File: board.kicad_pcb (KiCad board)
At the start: 2 copper layers, 135 x 100 mm, 12 parts, among them J1 Conn_01x02, J2 Conn_01x02, J3 Conn_01x02

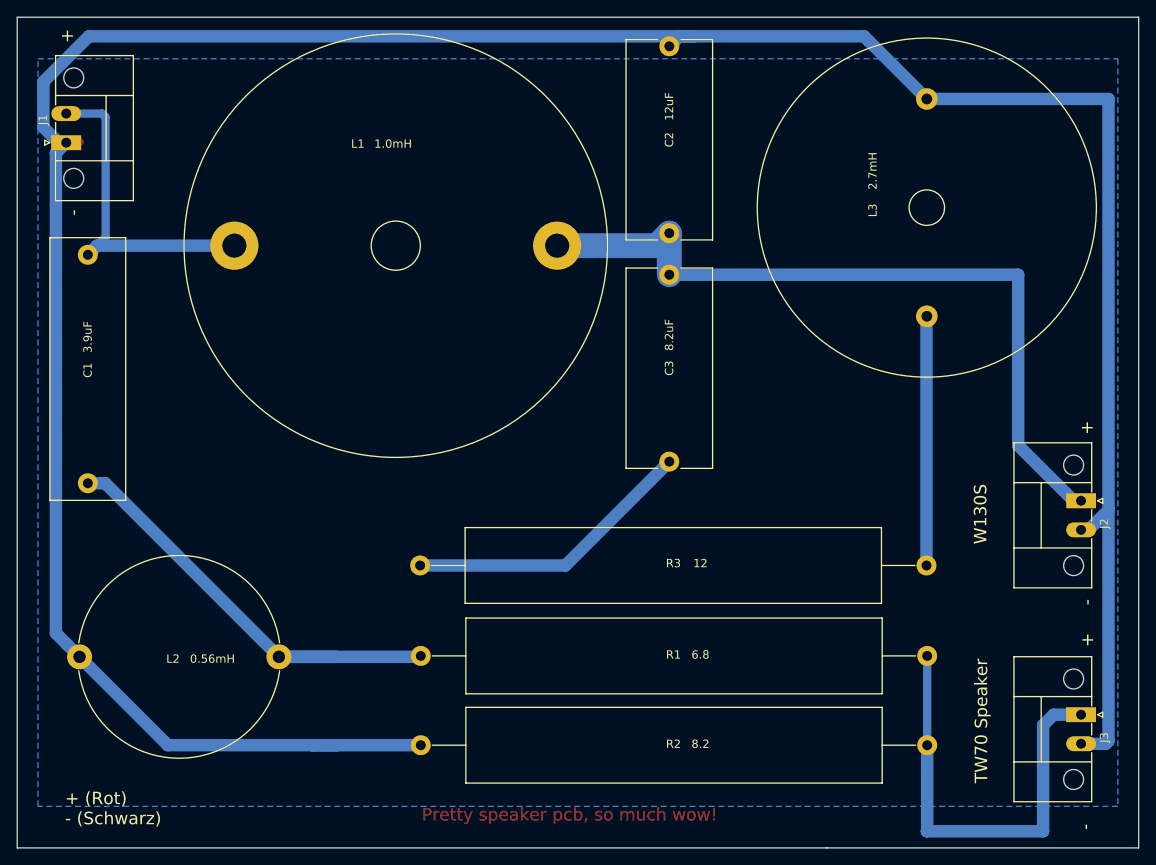
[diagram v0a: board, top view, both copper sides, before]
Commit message: Syncing AISLER project with GitHub repository
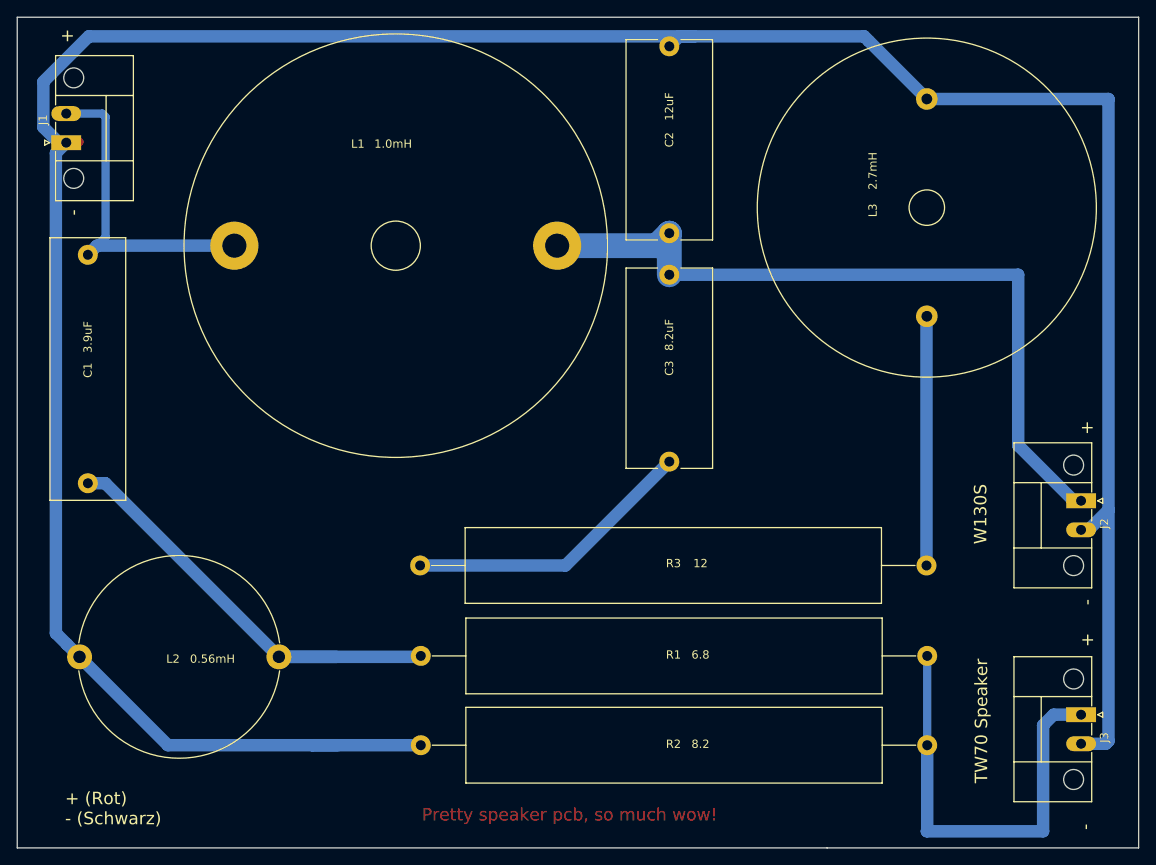
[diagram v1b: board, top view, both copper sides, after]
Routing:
- removed copper zone on B.Cu, net (none)
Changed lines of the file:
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@@
   (segment (start 124.5 82.5) (end 126 81) (width 3) (layer B.Cu) (net 7))
   (segment (start 126 86) (end 126 81) (width 3) (layer B.Cu) (net 7))
-  (zone (net 0) (net_name "") (layer B.Cu) (hatch edge 0.508)
-    (connect_pads (clearance 0.508))
-    (min_thickness 0.254)
-    (fill yes (arc_segments 16) (thermal_gap 0.508) (thermal_bridge_width 0.508))
-    (polygon
-      (pts
-        (xy 50 60) (xy 180 60) (xy 180 150) (xy 50 150)
-      )
-    )
-  )
 )

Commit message: Syncing AISLER project with GitHub repository
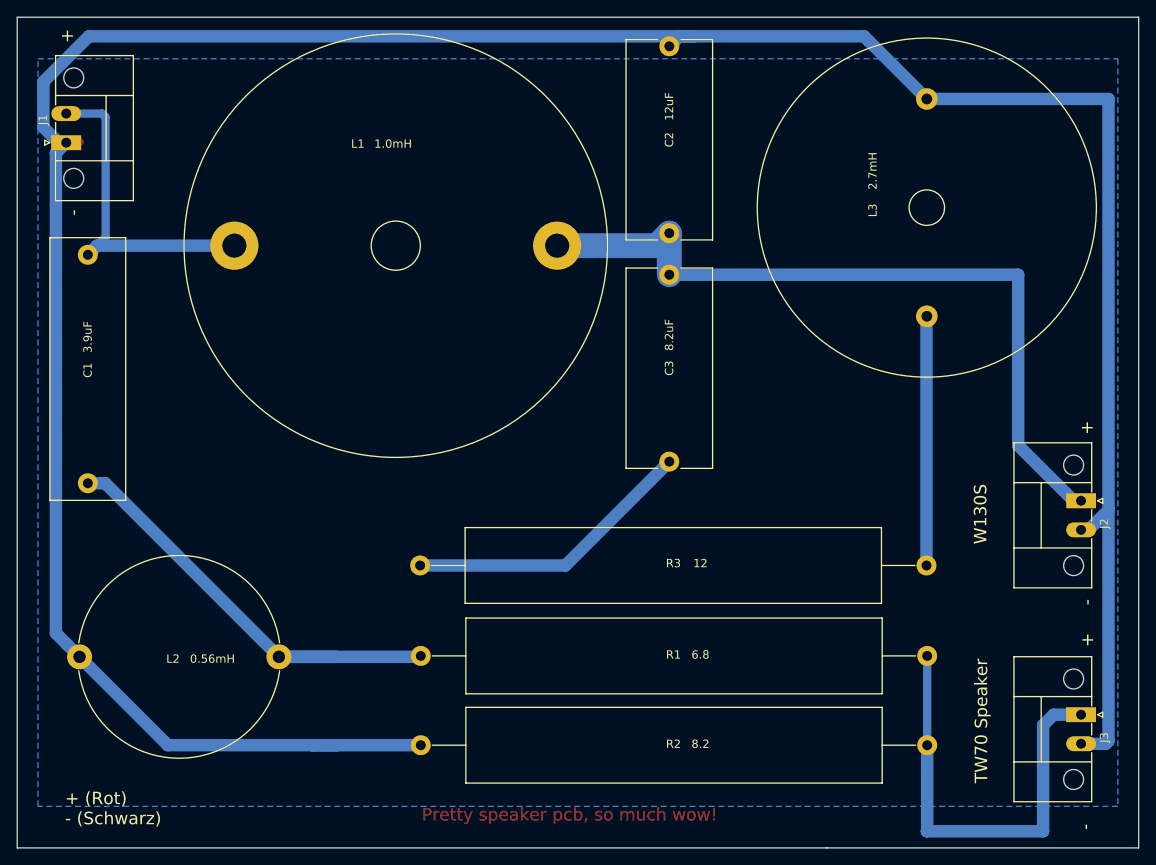
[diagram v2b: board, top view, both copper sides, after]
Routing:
- added copper zone on B.Cu, net (none)
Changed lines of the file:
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@@
   (segment (start 124.5 82.5) (end 126 81) (width 3) (layer B.Cu) (net 7))
   (segment (start 126 86) (end 126 81) (width 3) (layer B.Cu) (net 7))
+  (zone (net 0) (net_name "") (layer B.Cu) (hatch edge 0.508)
+    (connect_pads (clearance 0.508))
+    (min_thickness 0.254)
+    (fill yes (arc_segments 16) (thermal_gap 0.508) (thermal_bridge_width 0.508))
+    (polygon
+      (pts
+        (xy 50 60) (xy 180 60) (xy 180 150) (xy 50 150)
+      )
+    )
+  )
 )
